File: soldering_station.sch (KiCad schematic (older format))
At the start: 71 parts, among them IC1 ATMEGA8A-P, K1 dec in, K2 dec out, P1 17v, P10 disp in, P2 220v, P3 24v|220v, P4 solder, P5 thermocouple, P6 Fan, P7 thermocouple, P8 Heater, P9 disp out, Q1 КТ313Б, Q2 КТ313Б, Q3 КТ313Б, Q4 КТ815А, SW2 Enc, U1 TL072, U2 MOC3023M, U3 MOC3023M, U4 LM7805CT

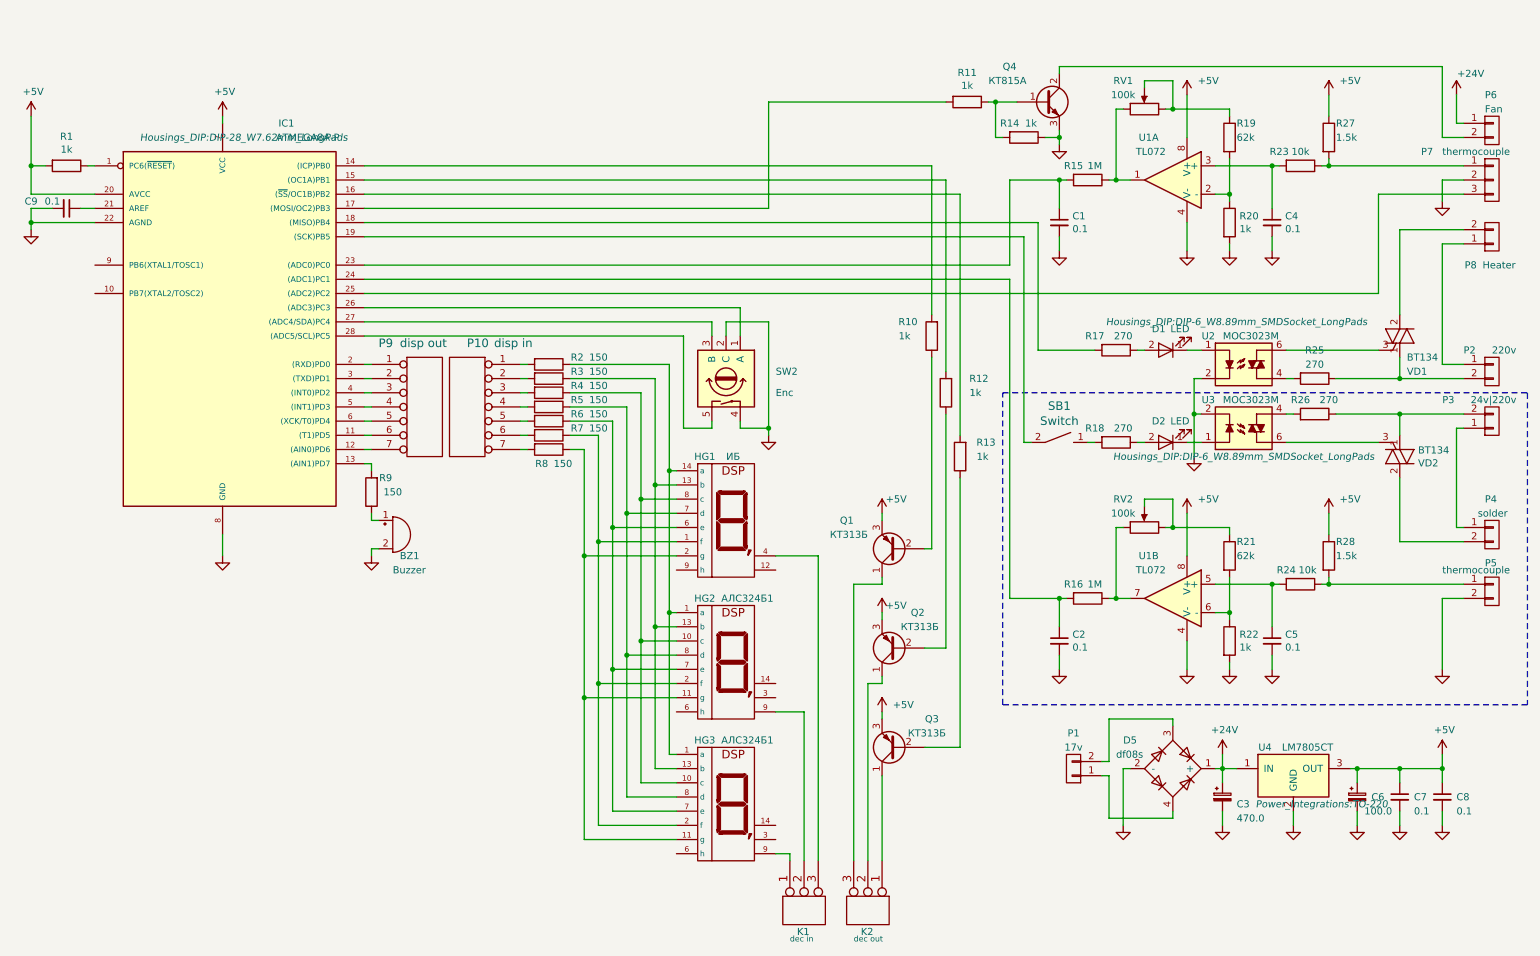
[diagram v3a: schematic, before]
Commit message: Display PCB
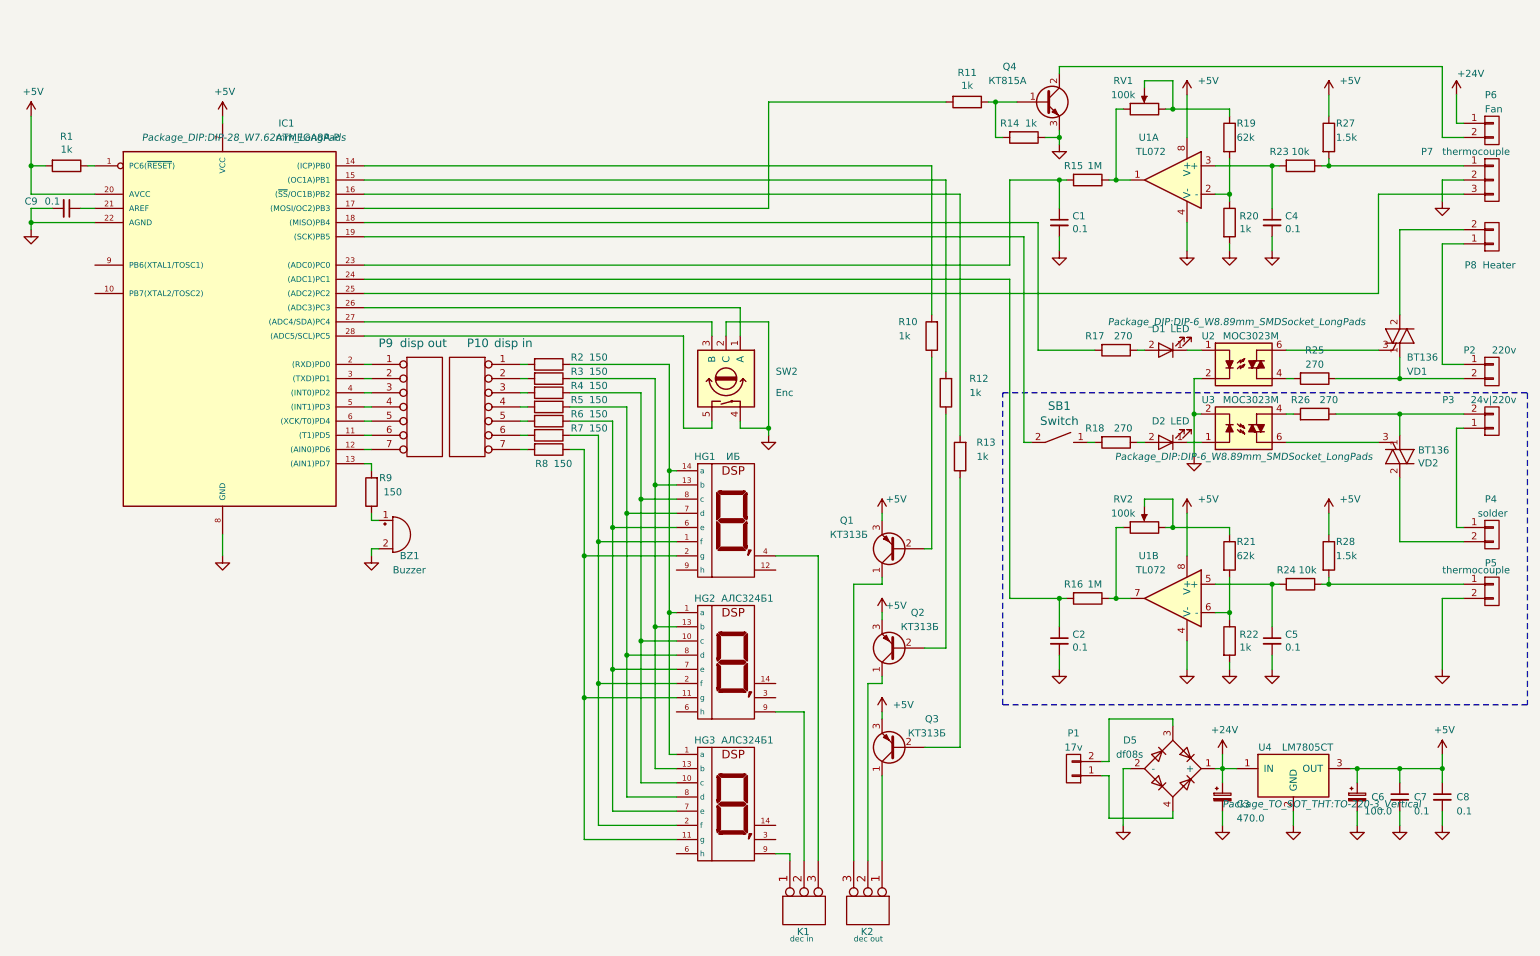
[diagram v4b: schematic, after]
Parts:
- BZ1: footprint Buzzers_Beepers:Buzzer_12x9.5RM7.6 -> Buzzer_Beeper:Buzzer_12x9.5RM7.6
- C1, C2, C4, C5, C7, C8, C9: footprint Capacitors_SMD:C_0805 -> Capacitor_SMD:C_0805_2012Metric
- C3: footprint Capacitors_ThroughHole:CP_Radial_D8.0mm_P3.80mm -> Capacitor_THT:CP_Radial_D8.0mm_P3.80mm
- C6: footprint Capacitors_ThroughHole:CP_Radial_D5.0mm_P2.50mm -> Capacitor_THT:CP_Radial_D5.0mm_P2.50mm
- D1, D2: footprint LEDs:LED_D5.0mm -> LED_THT:LED_D5.0mm
- D5: footprint Oscillators:Oscillator_SMD_SeikoEpson_SG8002JA-4pin_14.0x8.7mm -> Oscillator:Oscillator_SMD_SeikoEpson_SG8002JA-4Pin_14.0x8.7mm
- HG1: footprint Displays_7-Segment:MAN3640A -> lib:иб
- HG2, HG3: footprint Housings_DIP:DIP-14_W7.62mm_LongPads -> Package_DIP:DIP-14_W7.62mm
- IC1: footprint Housings_DIP:DIP-28_W7.62mm_LongPads -> Package_DIP:DIP-28_W7.62mm_LongPads
- K1, K2, P7: footprint Pin_Headers:Pin_Header_Straight_1x03_Pitch2.54mm -> Connector_PinHeader_2.54mm:PinHeader_1x03_P2.54mm_Vertical
- P1, P5, P6, SB1: footprint Pin_Headers:Pin_Header_Straight_1x02_Pitch2.54mm -> Connector_PinHeader_2.54mm:PinHeader_1x02_P2.54mm_Vertical
- P10, P9: footprint Pin_Headers:Pin_Header_Straight_1x07_Pitch2.54mm -> Connector_PinHeader_2.54mm:PinHeader_1x07_P2.54mm_Vertical
- P2, P3, P4, P8: footprint Pin_Headers:Pin_Header_Straight_1x02_Pitch3.96mm_Friction_Lock -> Connector_Wire:SolderWirePad_1x02_P5.08mm_Drill1.5mm
- Q1, Q2: footprint TO_SOT_Packages_THT:TO-92_Molded_Wide_Oval -> Package_TO_SOT_THT:TO-92L_Wide
- Q3: footprint TO_SOT_Packages_THT:TO-92_Molded_Wide_Oval -> Package_TO_SOT_THT:TO-92_Wide
- Q4: footprint TO_SOT_Packages_THT:TO-126_Vertical -> Package_TO_SOT_THT:TO-126-3_Vertical
- R1, R10, R11, R12, R13, R14, R15, R16, R17, R18, R19, R2, R20, R21, R22, R23, R24, R25, R26, R27, R28, R3, R4, R5, R6, R7, R8, R9: footprint Resistors_SMD:R_0805 -> Resistor_SMD:R_0805_2012Metric
- RV1, RV2: footprint Potentiometers:Potentiometer_Trimmer_ACP_CA9v_Horizontal_Px10.0mm_Py5.0mm -> Potentiometer_THT:Potentiometer_ACP_CA9-V10_Vertical
- SW2: footprint lib:Encoder_with_button -> Connector_PinHeader_2.54mm:PinHeader_1x05_P2.54mm_Vertical
- U1: footprint Housings_DIP:DIP-8_W8.89mm_SMDSocket_LongPads -> Package_DIP:DIP-8_W8.89mm_SMDSocket_LongPads
- U2, U3: footprint Housings_DIP:DIP-6_W8.89mm_SMDSocket_LongPads -> Package_DIP:DIP-6_W8.89mm_SMDSocket_LongPads
- U4: footprint Power_Integrations:TO-220 -> Package_TO_SOT_THT:TO-220-3_Vertical
- VD1, VD2: value BT134 -> BT136; footprint lib:sot82 -> Package_TO_SOT_THT:TO-220-3_Vertical

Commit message: Update PCB
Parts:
- BZ1: symbol soldering_station-rescue:Buzzer-soldering_station-rescue -> soldering_station-rescue:Buzzer-soldering_station-rescue-soldering_station-rescue
- C3, C6: symbol soldering_station-rescue:CP_Small-soldering_station-rescue -> soldering_station-rescue:CP_Small-soldering_station-rescue-soldering_station-rescue
- D1, D2: symbol soldering_station-rescue:LED-soldering_station-rescue -> soldering_station-rescue:LED-soldering_station-rescue-soldering_station-rescue
- D5: symbol soldering_station-rescue:D_Bridge_+-AA-soldering_station-rescue -> soldering_station-rescue:D_Bridge_+-AA-soldering_station-rescue-soldering_station-rescue
- HG1: symbol soldering_station-rescue:ИБ-иб -> soldering_station-rescue:ИБ-иб-soldering_station-rescue
- HG2, HG3: symbol soldering_station-rescue:АЛС324Б1-алс324б1 -> soldering_station-rescue:АЛС324Б1-алс324б1-soldering_station-rescue
- IC1: symbol soldering_station-rescue:ATMEGA8A-P-atmel -> soldering_station-rescue:ATMEGA8A-P-atmel-soldering_station-rescue
- K1, K2: symbol soldering_station-rescue:CONN_3-conn -> soldering_station-rescue:CONN_3-conn-soldering_station-rescue
- P1, P2, P3, P4, P5, P6, P8: symbol soldering_station-rescue:CONN_01X02-soldering_station-rescue -> soldering_station-rescue:CONN_01X02-soldering_station-rescue-soldering_station-rescue
- P10, P9: symbol soldering_station-rescue:CONN_7-conn -> soldering_station-rescue:CONN_7-conn-soldering_station-rescue
- P7: symbol soldering_station-rescue:CONN_01X03-soldering_station-rescue -> soldering_station-rescue:CONN_01X03-soldering_station-rescue-soldering_station-rescue
- Q1, Q2, Q3: symbol soldering_station-rescue:Q_PNP_CBE-soldering_station-rescue -> soldering_station-rescue:Q_PNP_CBE-soldering_station-rescue-soldering_station-rescue
- Q4: symbol soldering_station-rescue:Q_NPN_BCE-soldering_station-rescue -> soldering_station-rescue:Q_NPN_BCE-soldering_station-rescue-soldering_station-rescue
- SB1: symbol soldering_station-rescue:Switch-switch -> soldering_station-rescue:Switch-switch-soldering_station-rescue
- SW2: symbol soldering_station-rescue:Rotary_Encoder_Switch-soldering_station-rescue -> soldering_station-rescue:Rotary_Encoder_Switch-soldering_station-rescue-soldering_station-rescue
- U2, U3: symbol soldering_station-rescue:MOC3023M-soldering_station-rescue -> soldering_station-rescue:MOC3023M-soldering_station-rescue-soldering_station-rescue
- U4: symbol soldering_station-rescue:LM7805CT-soldering_station-rescue -> soldering_station-rescue:LM7805CT-soldering_station-rescue-soldering_station-rescue
- VD1, VD2: symbol soldering_station-rescue:BT139-bt139 -> soldering_station-rescue:BT139-bt139-soldering_station-rescue
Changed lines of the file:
@@
 $EndComp
 $Comp
-L soldering_station-rescue:ATMEGA8A-P-atmel IC1
+L soldering_station-rescue:ATMEGA8A-P-atmel-soldering_station-rescue IC1
 U 1 1 5912C25D
 P 1950 2400
@@
 $EndComp
 $Comp
-L soldering_station-rescue:Buzzer-soldering_station-rescue BZ1
+L soldering_station-rescue:Buzzer-soldering_station-rescue-soldering_station-rescue BZ1
 U 1 1 5913130E
 P 3150 3900
@@
 $EndComp
 $Comp
-L soldering_station-rescue:MOC3023M-soldering_station-rescue U2
+L soldering_station-rescue:MOC3023M-soldering_station-rescue-soldering_station-rescue U2
 U 1 1 59143D58
 P 9150 2700
@@
 $EndComp
 $Comp
-L soldering_station-rescue:MOC3023M-soldering_station-rescue U3
+L soldering_station-rescue:MOC3023M-soldering_station-rescue-soldering_station-rescue U3
 U 1 1 59143E30
 P 9150 3150
@@
 $EndComp
 $Comp
-L soldering_station-rescue:BT139-bt139 VD1
+L soldering_station-rescue:BT139-bt139-soldering_station-rescue VD1
 U 1 1 59145DE9
 P 10250 2500
@@
 $EndComp
 $Comp
-L soldering_station-rescue:BT139-bt139 VD2
+L soldering_station-rescue:BT139-bt139-soldering_station-rescue VD2
 U 1 1 59145E5D
 P 10250 3350
@@
 $EndComp
 $Comp
-L soldering_station-rescue:LED-soldering_station-rescue D1
+L soldering_station-rescue:LED-soldering_station-rescue-soldering_station-rescue D1
 U 1 1 59146F29
 P 8600 2600
@@
 $EndComp
 $Comp
-L soldering_station-rescue:LED-soldering_station-rescue D2
+L soldering_station-rescue:LED-soldering_station-rescue-soldering_station-rescue D2
 U 1 1 59147091
 P 8600 3250
@@
 $EndComp
 $Comp
-L soldering_station-rescue:CONN_01X02-soldering_station-rescue P2
+L soldering_station-rescue:CONN_01X02-soldering_station-rescue-soldering_station-rescue P2
 U 1 1 5914C58F
 P 10900 2750
@@
 $EndComp
 $Comp
-L soldering_station-rescue:CONN_01X02-soldering_station-rescue P3
+L soldering_station-rescue:CONN_01X02-soldering_station-rescue-soldering_station-rescue P3
 U 1 1 5914D402
 P 10900 3100
@@
 $EndComp
 $Comp
-L soldering_station-rescue:Switch-switch SB1
+L soldering_station-rescue:Switch-switch-soldering_station-rescue SB1
 U 1 1 5914E255
 P 7850 3250
@@
 $EndComp
 $Comp
-L soldering_station-rescue:CONN_01X02-soldering_station-rescue P4
+L soldering_station-rescue:CONN_01X02-soldering_station-rescue-soldering_station-rescue P4
 U 1 1 5914FDDB
 P 10900 3900
@@
 $EndComp
 $Comp
-L soldering_station-rescue:CONN_01X02-soldering_station-rescue P5
+L soldering_station-rescue:CONN_01X02-soldering_station-rescue-soldering_station-rescue P5
 U 1 1 5914FEAB
 P 10900 4300
@@
 $EndComp
 $Comp
-L soldering_station-rescue:Q_NPN_BCE-soldering_station-rescue Q4
+L soldering_station-rescue:Q_NPN_BCE-soldering_station-rescue-soldering_station-rescue Q4
 U 1 1 5916DF03
 P 7750 850
@@
 $EndComp
 $Comp
-L soldering_station-rescue:LM7805CT-soldering_station-rescue U4
+L soldering_station-rescue:LM7805CT-soldering_station-rescue-soldering_station-rescue U4
 U 1 1 5916F3BD
 P 9500 5600
@@
 $EndComp
 $Comp
-L soldering_station-rescue:CP_Small-soldering_station-rescue C6
+L soldering_station-rescue:CP_Small-soldering_station-rescue-soldering_station-rescue C6
 U 1 1 5916FF84
 P 9950 5750
@@
 $EndComp
 $Comp
-L soldering_station-rescue:CP_Small-soldering_station-rescue C3
+L soldering_station-rescue:CP_Small-soldering_station-rescue-soldering_station-rescue C3
 U 1 1 591704BF
 P 9000 5750
@@
 $EndComp
 $Comp
-L soldering_station-rescue:АЛС324Б1-алс324б1 HG2
+L soldering_station-rescue:АЛС324Б1-алс324б1-soldering_station-rescue HG2
 U 1 1 5919A435
 P 5550 4800
@@
 $EndComp
 $Comp
-L soldering_station-rescue:АЛС324Б1-алс324б1 HG3
+L soldering_station-rescue:АЛС324Б1-алс324б1-soldering_station-rescue HG3
 U 1 1 5919A4F5
 P 5550 5800
@@
 $EndComp
 $Comp
-L soldering_station-rescue:ИБ-иб HG1
+L soldering_station-rescue:ИБ-иб-soldering_station-rescue HG1
 U 1 1 5919A59F
 P 5550 3800
@@
 $EndComp
 $Comp
-L soldering_station-rescue:Q_PNP_CBE-soldering_station-rescue Q1
+L soldering_station-rescue:Q_PNP_CBE-soldering_station-rescue-soldering_station-rescue Q1
 U 1 1 591A31E1
 P 6700 4000
@@
 $EndComp
 $Comp
-L soldering_station-rescue:Q_PNP_CBE-soldering_station-rescue Q2
+L soldering_station-rescue:Q_PNP_CBE-soldering_station-rescue-soldering_station-rescue Q2
 U 1 1 591A32AD
 P 6700 4700
@@
 $EndComp
 $Comp
-L soldering_station-rescue:Q_PNP_CBE-soldering_station-rescue Q3
+L soldering_station-rescue:Q_PNP_CBE-soldering_station-rescue-soldering_station-rescue Q3
 U 1 1 591A334F
 P 6700 5400
@@
 $EndComp
 $Comp
-L soldering_station-rescue:D_Bridge_+-AA-soldering_station-rescue D5
+L soldering_station-rescue:D_Bridge_+-AA-soldering_station-rescue-soldering_station-rescue D5
 U 1 1 591D2084
 P 8650 5550
@@
 $EndComp
 $Comp
-L soldering_station-rescue:CONN_01X02-soldering_station-rescue P1
+L soldering_station-rescue:CONN_01X02-soldering_station-rescue-soldering_station-rescue P1
 U 1 1 591D2FEC
 P 7950 5550
@@
 $EndComp
 $Comp
-L soldering_station-rescue:CONN_01X02-soldering_station-rescue P6
+L soldering_station-rescue:CONN_01X02-soldering_station-rescue-soldering_station-rescue P6
 U 1 1 5922F5D6
 P 10900 1050
@@
 $EndComp
 $Comp
-L soldering_station-rescue:CONN_01X02-soldering_station-rescue P8
+L soldering_station-rescue:CONN_01X02-soldering_station-rescue-soldering_station-rescue P8
 U 1 1 5922F6D0
 P 10900 1800
@@
 $EndComp
 $Comp
-L soldering_station-rescue:CONN_01X03-soldering_station-rescue P7
+L soldering_station-rescue:CONN_01X03-soldering_station-rescue-soldering_station-rescue P7
 U 1 1 5922F790
 P 10900 1400
@@
 $EndComp
 $Comp
-L soldering_station-rescue:Rotary_Encoder_Switch-soldering_station-rescue SW2
+L soldering_station-rescue:Rotary_Encoder_Switch-soldering_station-rescue-soldering_station-rescue SW2
 U 1 1 59883EF1
 P 5500 2800
@@
 	6950 1300 2950 1300
 $Comp
-L soldering_station-rescue:CONN_3-conn K2
+L soldering_station-rescue:CONN_3-conn-soldering_station-rescue K2
 U 1 1 5DE2CB58
 P 6500 6550
@@
 	6600 4250 6600 4200
 $Comp
-L soldering_station-rescue:CONN_3-conn K1
+L soldering_station-rescue:CONN_3-conn-soldering_station-rescue K1
 U 1 1 5DE67BB4
 P 6050 6550
@@
 	5950 6200 5950 6150
 $Comp
-L soldering_station-rescue:CONN_7-conn P10
+L soldering_station-rescue:CONN_7-conn-soldering_station-rescue P10
 U 1 1 5DF4D6C2
 P 3700 3000
@@
 	4050 3300 4100 3300
 $Comp
-L soldering_station-rescue:CONN_7-conn P9
+L soldering_station-rescue:CONN_7-conn-soldering_station-rescue P9
 U 1 1 5E0351E0
 P 3350 3000
